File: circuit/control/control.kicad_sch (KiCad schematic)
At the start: 33 parts, among them J1 Conn_01x02_Socket, J2 Conn_02x20_Row_Letter_Last, J3 Conn_02x20_Row_Letter_Last, Q1 2SC1815, Q2 2SC1815, Q3 2SC1815, Q4 2SC1815, Q5 2SC1815, SW1 SW_Push, U1 ESP32-DevKitC, U2 4digit_7seg_led

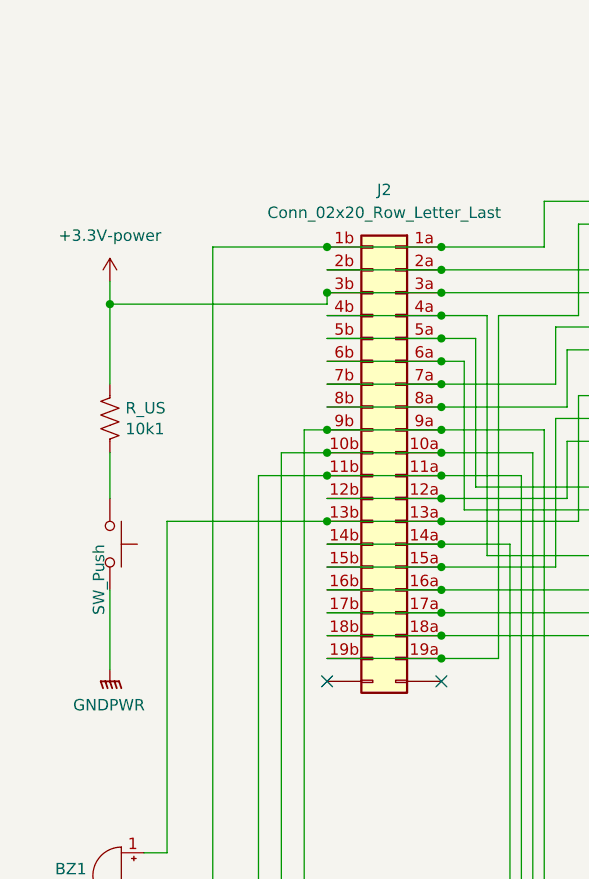
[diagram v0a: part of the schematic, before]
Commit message: [update] update control
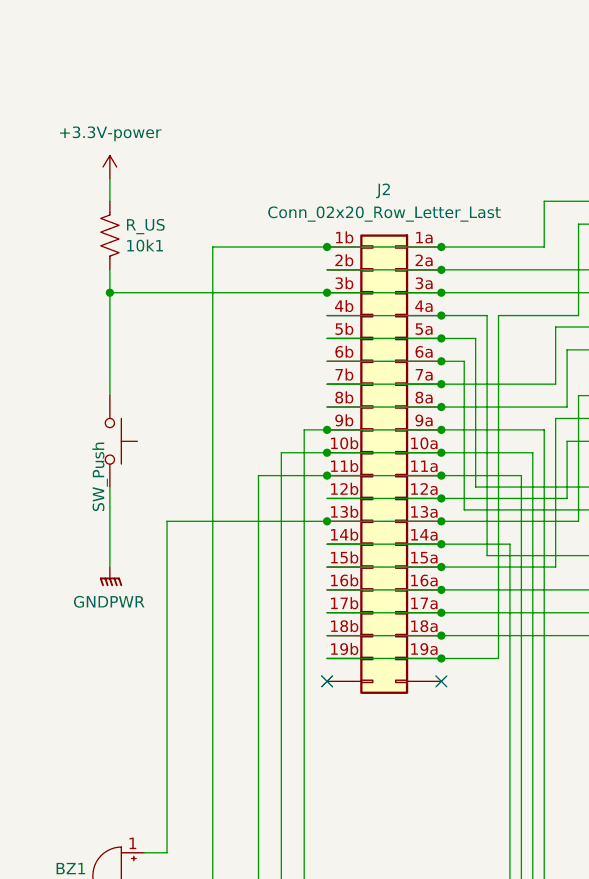
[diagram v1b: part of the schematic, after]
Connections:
- net +3V3: no longer J2.3a (Pin_3a), J2.3b (Pin_3b), U1.3 (SENSOR_VP/GPIO36/ADC1_CH0)
- net at 10k1.1, SW1.2: now also J2.3a (Pin_3a), J2.3b (Pin_3b), U1.3 (SENSOR_VP/GPIO36/ADC1_CH0)
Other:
- moved on the sheet: 10k1
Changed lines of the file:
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@@
   (junction (at 85.09 105.41) (diameter 0) (color 0 0 0 0)
   )
+  (junction (at 48.26 92.71) (diameter 0) (color 0 0 0 0)
+  )
   (junction (at 207.01 114.3) (diameter 0) (color 0 0 0 0)
   )
@@
   )
   (junction (at 138.43 78.74) (diameter 0) (color 0 0 0 0)
-  )
-  (junction (at 48.26 93.98) (diameter 0) (color 0 0 0 0)
   )
   (junction (at 85.09 128.27) (diameter 0) (color 0 0 0 0)
@@
     (stroke (width 0) (type default))
   )
-  (wire (pts (xy 48.26 91.44) (xy 48.26 93.98))
+  (wire (pts (xy 48.26 80.01) (xy 48.26 82.55))
     (stroke (width 0) (type default))
   )
@@
     (stroke (width 0) (type default))
   )
-  (wire (pts (xy 48.26 125.73) (xy 48.26 134.62))
+  (wire (pts (xy 48.26 114.3) (xy 48.26 123.19))
     (stroke (width 0) (type default))
   )
@@
     (stroke (width 0) (type default))
   )
-  (wire (pts (xy 72.39 93.98) (xy 72.39 92.71))
-    (stroke (width 0) (type default))
-  )
   (wire (pts (xy 191.77 123.19) (xy 191.77 168.91))
     (stroke (width 0) (type default))
@@
     (stroke (width 0) (type default))
   )
-  (wire (pts (xy 48.26 110.49) (xy 48.26 115.57))
+  (wire (pts (xy 48.26 90.17) (xy 48.26 92.71))
     (stroke (width 0) (type default))
   )
@@
     (stroke (width 0) (type default))
   )
-  (wire (pts (xy 48.26 93.98) (xy 48.26 102.87))
-    (stroke (width 0) (type default))
-  )
   (wire (pts (xy 254 180.34) (xy 254 184.15))
     (stroke (width 0) (type default))
@@
     (stroke (width 0) (type default))
   )
+  (wire (pts (xy 48.26 92.71) (xy 48.26 104.14))
+    (stroke (width 0) (type default))
+  )
   (wire (pts (xy 243.84 104.14) (xy 243.84 151.13))
     (stroke (width 0) (type default))
@@
     (stroke (width 0) (type default))
   )
-  (wire (pts (xy 48.26 93.98) (xy 72.39 93.98))
-    (stroke (width 0) (type default))
-  )
   (wire (pts (xy 228.6 119.38) (xy 246.38 119.38))
     (stroke (width 0) (type default))
@@
   )
   (wire (pts (xy 189.23 120.65) (xy 171.45 120.65))
+    (stroke (width 0) (type default))
+  )
+  (wire (pts (xy 48.26 92.71) (xy 72.39 92.71))
     (stroke (width 0) (type default))
   )
@@
     )
   )
-  (symbol (lib_id "power:GNDPWR") (at 48.26 134.62 0) (mirror y) (unit 1)
-    (in_bom yes) (on_board yes) (dnp no)
-    (property "Reference" "#PWR02" (at 48.26 139.7 0)
-      (effects (font (size 1.27 1.27)) hide)
-    )
-    (property "Value" "GNDPWR" (at 48.1584 138.5316 0)
+  (symbol (lib_id "power:GNDPWR") (at 48.26 123.19 0) (mirror y) (unit 1)
+    (in_bom yes) (on_board yes) (dnp no)
+    (property "Reference" "#PWR02" (at 48.26 128.27 0)
+      (effects (font (size 1.27 1.27)) hide)
+    )
+    (property "Value" "GNDPWR" (at 48.1584 127.1016 0)
       (effects (font (size 1.27 1.27)))
     )
-    (property "Footprint" "" (at 48.26 135.89 0)
-      (effects (font (size 1.27 1.27)) hide)
-    )
-    (property "Datasheet" "" (at 48.26 135.89 0)
+    (property "Footprint" "" (at 48.26 124.46 0)
+      (effects (font (size 1.27 1.27)) hide)
+    )
+    (property "Datasheet" "" (at 48.26 124.46 0)
       (effects (font (size 1.27 1.27)) hide)
     )
@@
     )
   )
-  (symbol (lib_id "Device:R_US") (at 48.26 106.68 0) (mirror x) (unit 1)
-    (in_bom yes) (on_board yes) (dnp no)
-    (property "Reference" "10k1" (at 49.9872 107.8484 0)
+  (symbol (lib_id "Device:R_US") (at 48.26 86.36 0) (mirror x) (unit 1)
+    (in_bom yes) (on_board yes) (dnp no)
+    (property "Reference" "10k1" (at 49.9872 87.5284 0)
       (effects (font (size 1.27 1.27)) (justify left))
     )
-    (property "Value" "R_US" (at 49.9872 105.537 0)
+    (property "Value" "R_US" (at 49.9872 85.217 0)
       (effects (font (size 1.27 1.27)) (justify left))
     )
-    (property "Footprint" "Resistor_THT:R_Axial_DIN0207_L6.3mm_D2.5mm_P10.16mm_Horizontal" (at 49.276 106.426 90)
-      (effects (font (size 1.27 1.27)) hide)
-    )
-    (property "Datasheet" "~" (at 48.26 106.68 0)
+    (property "Footprint" "Resistor_THT:R_Axial_DIN0207_L6.3mm_D2.5mm_P10.16mm_Horizontal" (at 49.276 86.106 90)
+      (effects (font (size 1.27 1.27)) hide)
+    )
+    (property "Datasheet" "~" (at 48.26 86.36 0)
       (effects (font (size 1.27 1.27)) hide)
     )
@@
     )
   )
-  (symbol (lib_id "Switch:SW_Push") (at 48.26 120.65 270) (mirror x) (unit 1)
-    (in_bom yes) (on_board yes) (dnp no)
-    (property "Reference" "SW1" (at 55.499 120.65 0)
-      (effects (font (size 1.27 1.27)) hide)
-    )
-    (property "Value" "SW_Push" (at 47.0408 120.65 0)
+  (symbol (lib_id "Switch:SW_Push") (at 48.26 109.22 270) (mirror x) (unit 1)
+    (in_bom yes) (on_board yes) (dnp no)
+    (property "Reference" "SW1" (at 55.499 109.22 0)
+      (effects (font (size 1.27 1.27)) hide)
+    )
+    (property "Value" "SW_Push" (at 47.0408 109.22 0)
       (effects (font (size 1.27 1.27)) (justify right))
     )
-    (property "Footprint" "Button_Switch_THT:SW_PUSH-12mm_Wuerth-430476085716" (at 53.34 120.65 0)
-      (effects (font (size 1.27 1.27)) hide)
-    )
-    (property "Datasheet" "~" (at 53.34 120.65 0)
+    (property "Footprint" "Button_Switch_THT:SW_PUSH-12mm_Wuerth-430476085716" (at 53.34 109.22 0)
+      (effects (font (size 1.27 1.27)) hide)
+    )
+    (property "Datasheet" "~" (at 53.34 109.22 0)
       (effects (font (size 1.27 1.27)) hide)
     )
@@
     )
   )
-  (symbol (lib_id "control-rescue:+3.3V-power") (at 48.26 91.44 0) (mirror y) (unit 1)
+  (symbol (lib_id "control-rescue:+3.3V-power") (at 48.26 80.01 0) (mirror y) (unit 1)
     (in_bom yes) (on_board yes) (dnp no) (fields_autoplaced)
-    (property "Reference" "#PWR01" (at 48.26 95.25 0)
-      (effects (font (size 1.27 1.27)) hide)
-    )
-    (property "Value" "+3.3V-power" (at 48.26 86.36 0)
+    (property "Reference" "#PWR01" (at 48.26 83.82 0)
+      (effects (font (size 1.27 1.27)) hide)
+    )
+    (property "Value" "+3.3V-power" (at 48.26 74.93 0)
       (effects (font (size 1.27 1.27)))
     )
-    (property "Footprint" "" (at 48.26 91.44 0)
-      (effects (font (size 1.27 1.27)) hide)
-    )
-    (property "Datasheet" "" (at 48.26 91.44 0)
-      (effects (font (size 1.27 1.27)) hide)
-    )
+    (property "Footprint" "" (at 48.26 80.01 0)
+      (effects (font (size 1.27 1.27)) hide)
+    )
+    (property "Datasheet" "" (at 48.26 80.01 0)
+      (effects (font (size 1.27 1.27)) hide)
+    )
